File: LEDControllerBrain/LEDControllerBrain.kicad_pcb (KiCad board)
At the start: 2 copper layers, 10 parts, among them J1 TB001-500-04BE, J2 TB001-500-04BE, J3 TB001-500-04BE, U1 NODEMCU-32S

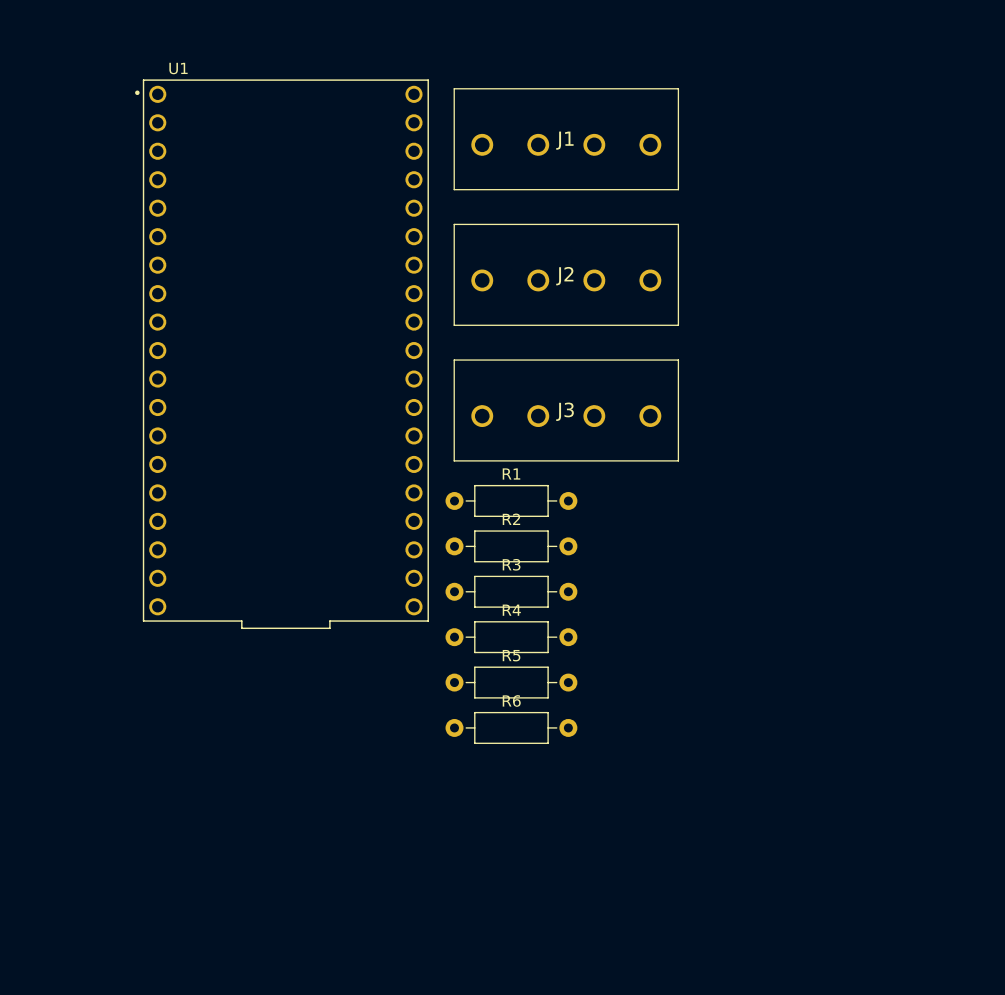
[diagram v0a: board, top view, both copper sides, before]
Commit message: done
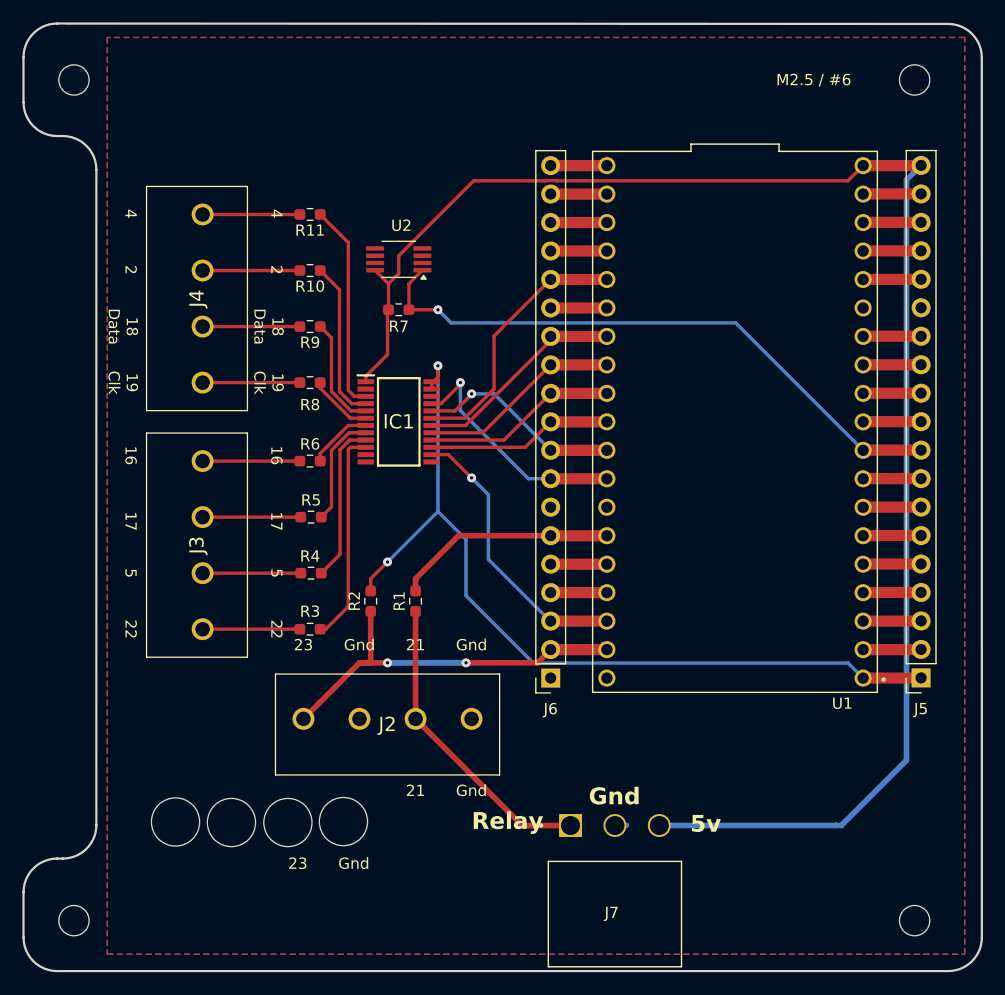
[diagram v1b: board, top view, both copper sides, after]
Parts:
- removed J1: TB001-500-04BE, LEDController:TB00150004BE
- added IC1: 74LVC4245APW,118, LEDController:SOP65P640X110-24N, F.Cu at (125.5, 89.5)
- added J4: TB001-500-04BE, LEDController:TB00150004BE, F.Cu at (108.0, 86.0)
- added J5: Conn_01x19_Pin, Connector_PinSocket_2.54mm:PinSocket_1x19_P2.54mm_Vertical, F.Cu at (172.1, 112.3)
- added J6: Conn_01x19_Pin, Connector_PinSocket_2.54mm:PinSocket_1x19_P2.54mm_Vertical, F.Cu at (139.1, 112.4)
- added J7: 647676-3, LEDController:TE_647676-3, F.Cu at (140.8, 125.5)
- added M2.5 / #6: MountingHole_2.7mm_M2.5, MountingHole:MountingHole_2.7mm_M2.5, F.Cu at (96.5, 59.0)
- added R10: 100, Resistor_SMD:R_0603_1608Metric_Pad0.98x0.95mm_HandSolder, F.Cu at (117.6, 76.0)
- added R11: 100, Resistor_SMD:R_0603_1608Metric_Pad0.98x0.95mm_HandSolder, F.Cu at (117.6, 71.0)
- added R7: 4.7k, Resistor_SMD:R_0603_1608Metric_Pad0.98x0.95mm_HandSolder, F.Cu at (125.5, 79.5)
- added R8: 100, Resistor_SMD:R_0603_1608Metric_Pad0.98x0.95mm_HandSolder, F.Cu at (117.6, 86.0)
- added R9: 100, Resistor_SMD:R_0603_1608Metric_Pad0.98x0.95mm_HandSolder, F.Cu at (117.6, 81.0)
- added REF**: MountingHole_4.3mm_M4, MountingHole:MountingHole_4.3mm_M4, F.Cu at (115.6, 125.2)
- added REF**: MountingHole_4.3mm_M4, MountingHole:MountingHole_4.3mm_M4, F.Cu at (105.6, 125.2)
- added REF**: MountingHole_4.3mm_M4, MountingHole:MountingHole_4.3mm_M4, F.Cu at (120.6, 125.2)
- added REF**: MountingHole_2.7mm_M2.5, MountingHole:MountingHole_2.7mm_M2.5, F.Cu at (96.5, 134.0)
- added REF**: MountingHole_2.7mm_M2.5, MountingHole:MountingHole_2.7mm_M2.5, F.Cu at (171.5, 59.0)
- added REF**: MountingHole_2.7mm_M2.5, MountingHole:MountingHole_2.7mm_M2.5, F.Cu at (171.5, 134.0)
- added REF**: MountingHole_4.3mm_M4, MountingHole:MountingHole_4.3mm_M4, F.Cu at (110.6, 125.2)
- added U2: DS18B20U, Package_SO:MSOP-8_3x3mm_P0.65mm, F.Cu at (125.5, 75.0)
- R1: value R -> 1k; footprint Resistor_THT:R_Axial_DIN0207_L6.3mm_D2.5mm_P10.16mm_Horizontal -> Resistor_SMD:R_0603_1608Metric_Pad0.98x0.95mm_HandSolder
- R2: value R -> 10k; footprint Resistor_THT:R_Axial_DIN0207_L6.3mm_D2.5mm_P10.16mm_Horizontal -> Resistor_SMD:R_0603_1608Metric_Pad0.98x0.95mm_HandSolder
- R3, R4, R5, R6: value R -> 100; footprint Resistor_THT:R_Axial_DIN0207_L6.3mm_D2.5mm_P10.16mm_Horizontal -> Resistor_SMD:R_0603_1608Metric_Pad0.98x0.95mm_HandSolder
- moved U1 40.6 mm to (155.5, 89.5), turned to 180 degrees
- moved J2 39.1 mm to (132.0, 116.0), turned to 180 degrees
- moved J3 31.4 mm to (108.0, 108.0), turned to 90 degrees
- moved R6 27.1 mm to (117.6, 93.0), turned to 180 degrees
- moved R5 19.5 mm to (117.7, 98.0), turned to 180 degrees
- moved R4 14.0 mm to (117.7, 103.0), turned to 180 degrees
- moved R3 13.3 mm to (117.6, 108.0), turned to 180 degrees
- moved R1 9.59 mm to (127.0, 105.5), turned to 90 degrees
- moved R2 8.93 mm to (123.0, 105.5), turned to 90 degrees
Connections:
- J2 pad 1: unconnected-(J2-Pad1) -> GND
- J2 pad 2: unconnected-(J2-Pad2) -> /Relay Controll
- J2 pad 3: unconnected-(J2-Pad3) -> GND
- J2 pad 4: unconnected-(J2-Pad4) -> /23
- J3 pad 1: unconnected-(J3-Pad1) -> Net-(J3-Pad1)
- J3 pad 2: unconnected-(J3-Pad2) -> Net-(J3-Pad2)
- J3 pad 3: unconnected-(J3-Pad3) -> Net-(J3-Pad3)
- J3 pad 4: unconnected-(J3-Pad4) -> Net-(J3-Pad4)
- R1 pad 1: unconnected-(R1-Pad1) -> /Relay Controll
- R1 pad 2: unconnected-(R1-Pad2) -> /21
- R2 pad 1: unconnected-(R2-Pad1) -> /23
- R2 pad 2: unconnected-(R2-Pad2) -> +3V3
- R3 pad 1: unconnected-(R3-Pad1) -> Net-(IC1-A7)
- R3 pad 2: unconnected-(R3-Pad2) -> Net-(J3-Pad1)
- R4 pad 1: unconnected-(R4-Pad1) -> Net-(IC1-A6)
- R4 pad 2: unconnected-(R4-Pad2) -> Net-(J3-Pad2)
- R5 pad 1: unconnected-(R5-Pad1) -> Net-(IC1-A5)
- R5 pad 2: unconnected-(R5-Pad2) -> Net-(J3-Pad3)
- R6 pad 2: Net-(U1-IO13) -> Net-(J3-Pad4)
- U1 pad J1_1: unconnected-(U1-3.3V-PadJ1_1) -> +3V3
- U1 pad J1_10: unconnected-(U1-IO26-PadJ1_10) -> /26
- U1 pad J1_11: unconnected-(U1-IO27-PadJ1_11) -> /27
- U1 pad J1_12: Net-(U1-IO14) -> /14
- U1 pad J1_13: unconnected-(U1-IO12-PadJ1_13) -> /12
- U1 pad J1_14: Net-(U1-GND-PadJ1_14) -> GND
- U1 pad J1_15: Net-(U1-IO13) -> /13
- U1 pad J1_16: unconnected-(U1-IO9-PadJ1_16) -> /9
- U1 pad J1_17: unconnected-(U1-IO10-PadJ1_17) -> /10
- U1 pad J1_18: unconnected-(U1-IO11-PadJ1_18) -> /11
- U1 pad J1_19: unconnected-(U1-5V-PadJ1_19) -> +5V
- U1 pad J1_2: unconnected-(U1-EN-PadJ1_2) -> /EN
- U1 pad J1_3: unconnected-(U1-IO36-PadJ1_3) -> /36
- U1 pad J1_4: unconnected-(U1-IO39-PadJ1_4) -> /39
- U1 pad J1_5: unconnected-(U1-IO34-PadJ1_5) -> /34
- U1 pad J1_6: unconnected-(U1-IO35-PadJ1_6) -> /35
- U1 pad J1_7: unconnected-(U1-IO32-PadJ1_7) -> /32
- U1 pad J1_8: unconnected-(U1-IO33-PadJ1_8) -> /33
- U1 pad J1_9: unconnected-(U1-IO25-PadJ1_9) -> /25
- U1 pad J2_1: Net-(U1-GND-PadJ1_14) -> GND
- U1 pad J2_10: unconnected-(U1-IO5-PadJ2_10) -> /5
- U1 pad J2_11: unconnected-(U1-IO17-PadJ2_11) -> /17
- U1 pad J2_12: unconnected-(U1-IO16-PadJ2_12) -> /16
- U1 pad J2_13: unconnected-(U1-IO4-PadJ2_13) -> /4
- U1 pad J2_14: unconnected-(U1-IO0-PadJ2_14) -> /0
- U1 pad J2_15: unconnected-(U1-IO2-PadJ2_15) -> /2
- U1 pad J2_16: unconnected-(U1-IO15-PadJ2_16) -> /15
- U1 pad J2_17: unconnected-(U1-IO8-PadJ2_17) -> /8
- U1 pad J2_18: unconnected-(U1-IO7-PadJ2_18) -> /7
- U1 pad J2_19: unconnected-(U1-IO6-PadJ2_19) -> /6
- U1 pad J2_2: unconnected-(U1-IO23-PadJ2_2) -> /23
- U1 pad J2_3: unconnected-(U1-IO22-PadJ2_3) -> /22
- U1 pad J2_4: unconnected-(U1-TX0-PadJ2_4) -> /1
- U1 pad J2_5: unconnected-(U1-RX0-PadJ2_5) -> /3
- U1 pad J2_6: unconnected-(U1-IO21-PadJ2_6) -> /21
- U1 pad J2_7: Net-(U1-GND-PadJ1_14) -> GND
- U1 pad J2_8: unconnected-(U1-IO19-PadJ2_8) -> /19
- U1 pad J2_9: unconnected-(U1-IO18-PadJ2_9) -> /18
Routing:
- net +5V: track 0.00 -> 142.2 mm
- net +3V3: track 0.00 -> 78.3 mm, vias 0 -> 2
- net /25: track 0.00 -> 54.9 mm, vias 0 -> 1
- net /23: track 0.00 -> 35.2 mm, vias 0 -> 2
- net /Relay Controll: track 0.00 -> 27.4 mm
- net /22: track 0.00 -> 25.2 mm, vias 0 -> 1
- net /2: track 0.00 -> 23.5 mm
- net /19: track 0.00 -> 21.5 mm, vias 0 -> 1
- net /21: track 0.00 -> 19.8 mm
- net /4: track 0.00 -> 19.1 mm
- net Net-(IC1-A7): track 0.00 -> 19.0 mm
- net Net-(IC1-A0): track 0.00 -> 18.5 mm
- net /18: track 0.00 -> 18.4 mm, vias 0 -> 1
- net /16: track 0.00 -> 18.1 mm
- net /17: track 0.00 -> 17.4 mm
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- added copper zone on B.Cu, net GND
- added copper zone on F.Cu, net GND
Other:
- board outline added: 85.5 x 84.5 mm
- board text added: "16"
- board text added: "17"
- board text added: "18 Data"
- board text added: "19 Clk"
- board text added: "2"
- board text added: "21"
- board text added: "22"
- board text added: "23"
- board text added: "4"
- board text added: "5"
- board text added: "5v"
- board text added: "Gnd"
- board text added: "Relay"
